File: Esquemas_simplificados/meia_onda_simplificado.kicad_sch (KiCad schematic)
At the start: 23 parts

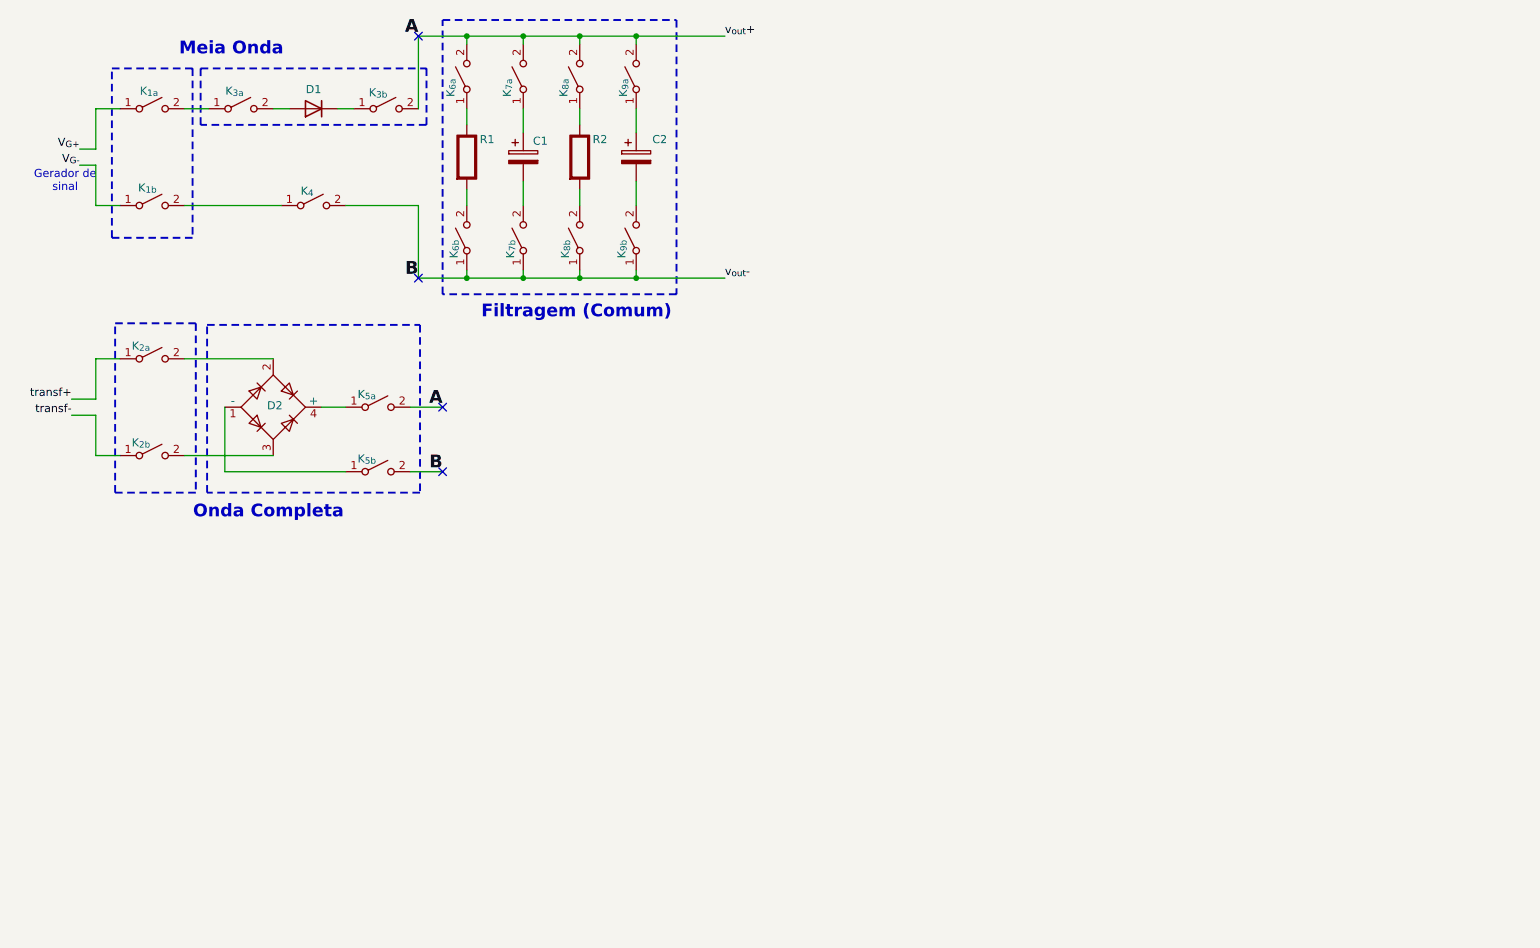
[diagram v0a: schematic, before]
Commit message: update chap 4 - filtros
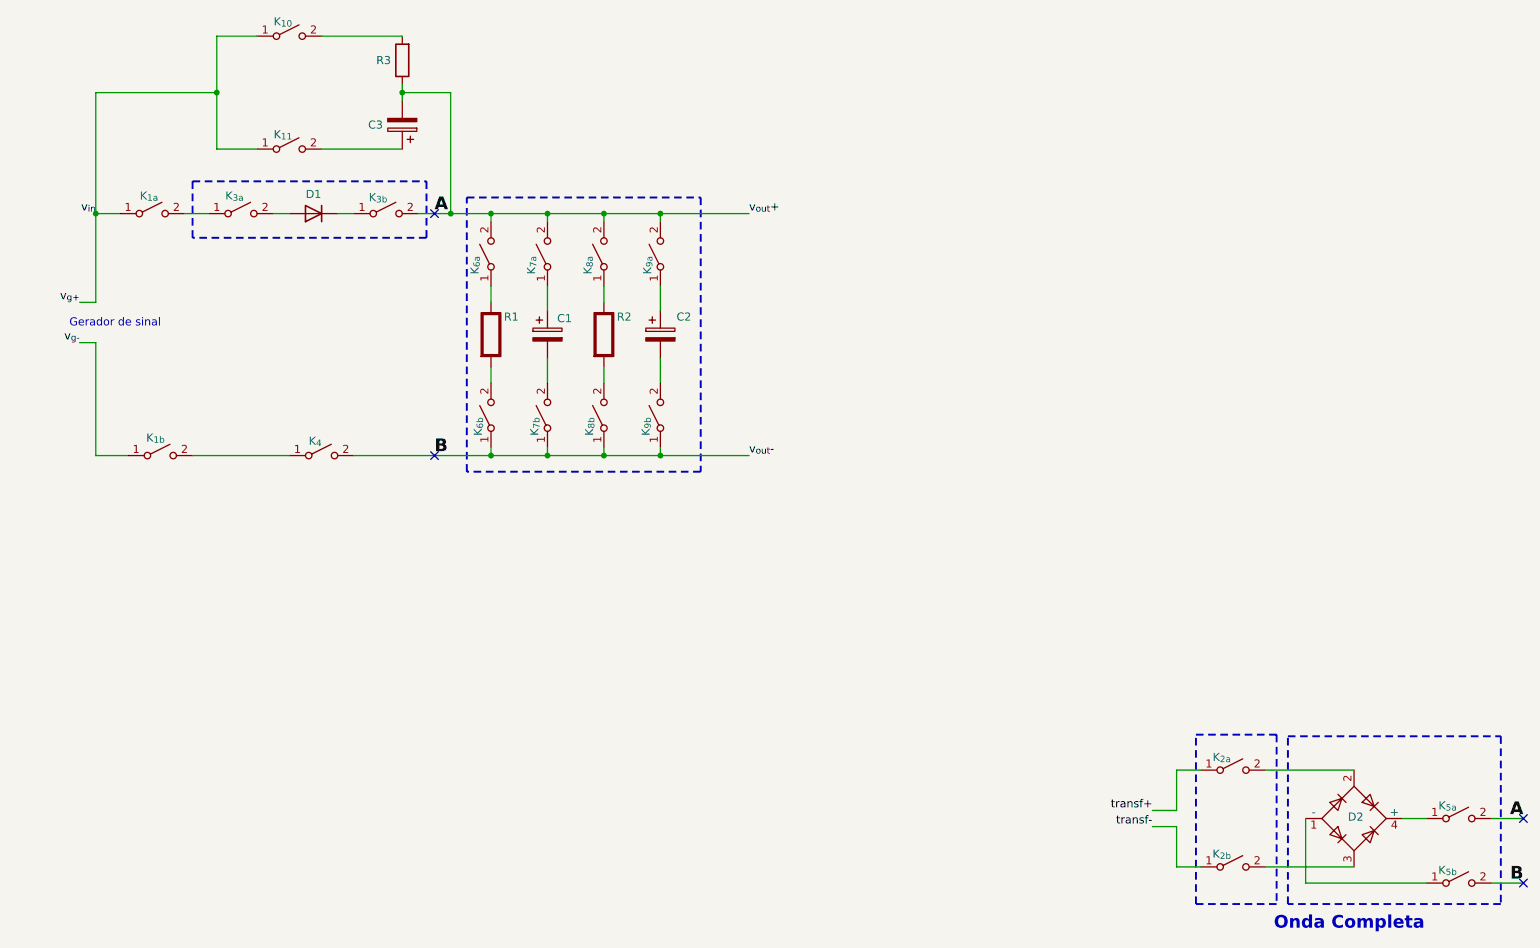
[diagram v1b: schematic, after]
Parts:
- added C3: 10uF, Capacitor_THT:CP_Radial_D5.0mm_P2.00mm, symbol Device:C_Polarized
- added K_{10}, K_{11}: SW_SPST, symbol Switch:SW_SPST
- added R3: 1K, Resistor_THT:R_Axial_DIN0207_L6.3mm_D2.5mm_P15.24mm_Horizontal, symbol Device:R
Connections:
- net A: now also C3.2, R3.1
- net V_{G+} renamed v_{g+}
- net v_{g+}: now also K_{10}.1 (A), K_{11}.1 (A)
- net V_{G-} renamed v_{g-}
- new net: K_{10}.2 (B), R3.2
- new net: C3.1, K_{11}.2 (B)
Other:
- note removed: "Filtragem (Comum)"
- note removed: "Meia Onda"
- moved on the sheet: C1, C2, D1, D2, K_{1a}, K_{1b}, K_{2a}, K_{2b}, K_{3a}, K_{3b}, K_{4}, K_{5a}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
